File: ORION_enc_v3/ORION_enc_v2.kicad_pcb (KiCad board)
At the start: 2 copper layers, 24 x 31 mm, 21 parts, among them J1 Conn_01x01, J2 Conn_01x01, J3 Conn_01x01, J4 Conn_01x01, J5 Conn_01x01, J6 Conn_01x01, J7 Conn_01x01, U1 AS5047D

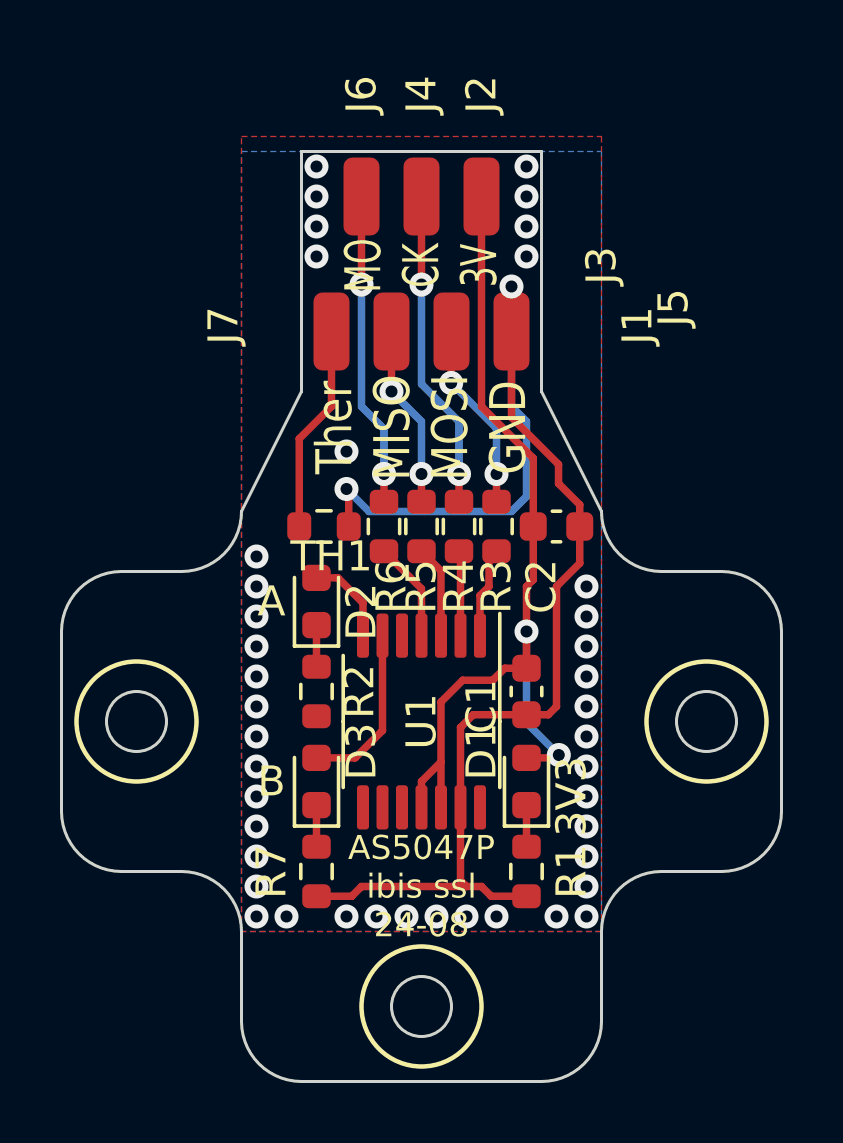
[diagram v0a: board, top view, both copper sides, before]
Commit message: 全てを追加
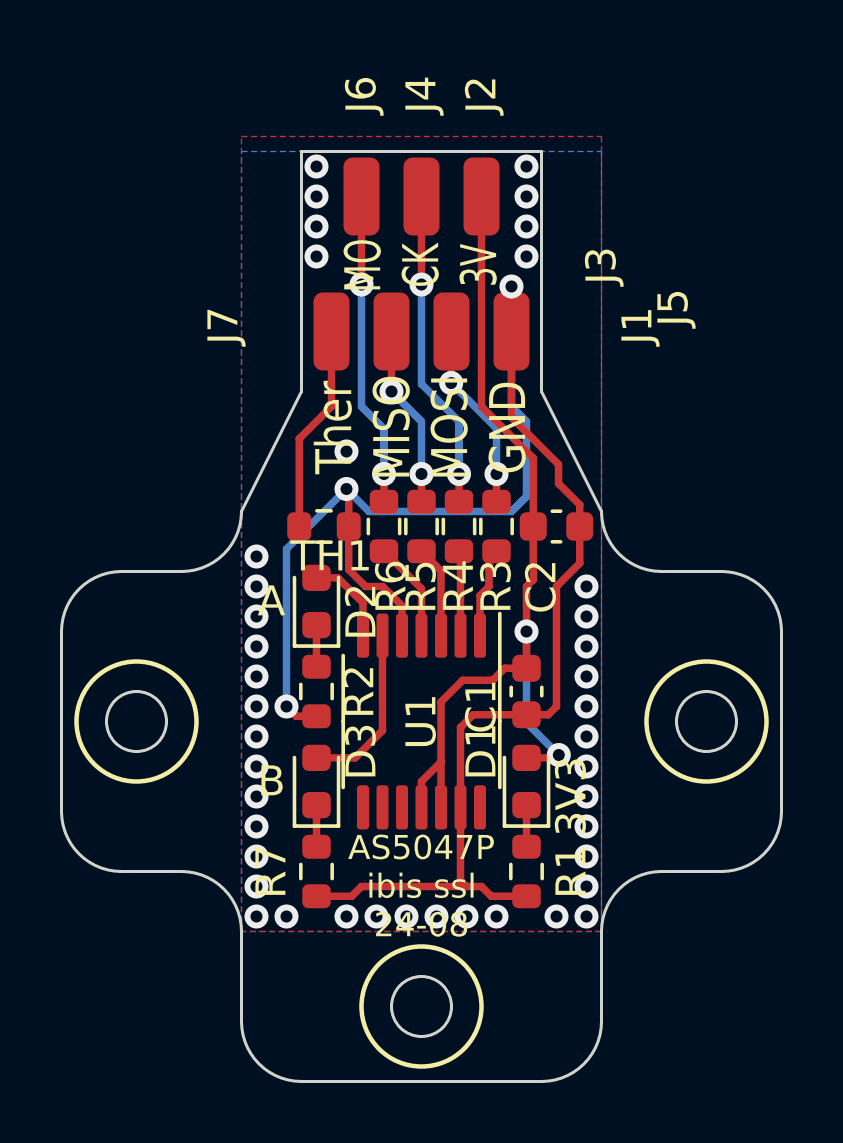
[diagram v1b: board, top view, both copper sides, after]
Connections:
- U1 pad 5: unconnected-(U1-Pad5) -> GND
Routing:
- net GND: track 46.7 -> 60.6 mm, vias 44 -> 45
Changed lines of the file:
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@@
   (net 12 "/MOSI")
   (net 13 "Net-(J7-Pad1)")
-  (net 14 "unconnected-(U1-Pad5)")
-  (net 15 "unconnected-(U1-Pad8)")
-  (net 16 "unconnected-(U1-Pad9)")
-  (net 17 "unconnected-(U1-Pad10)")
-  (net 18 "/OUT_A")
-  (net 19 "Net-(D3-Pad1)")
-  (net 20 "/OUT_B")
-  (net 21 "unconnected-(U1-Pad14)")
+  (net 14 "unconnected-(U1-Pad8)")
+  (net 15 "unconnected-(U1-Pad9)")
+  (net 16 "unconnected-(U1-Pad10)")
+  (net 17 "/OUT_A")
+  (net 18 "Net-(D3-Pad1)")
+  (net 19 "/OUT_B")
+  (net 20 "unconnected-(U1-Pad14)")
   (footprint "user:WireSoldingPad" (layer "F.Cu")
     (at 67 46.5 90)
@@
       (net 12 "/MOSI") (pinfunction "MOSI") (pintype "input"))
     (pad "5" smd roundrect (at -2.8625 0.65 270) (size 1.475 0.4) (layers "F.Cu" "F.Paste" "F.Mask") (roundrect_rratio 0.25)
-      (net 14 "unconnected-(U1-Pad5)") (pinfunction "TST") (pintype "input+no_connect"))
+      (net 2 "GND") (pinfunction "TST") (pintype "input"))
     (pad "6" smd roundrect (at -2.8625 1.3 270) (size 1.475 0.4) (layers "F.Cu" "F.Paste" "F.Mask") (roundrect_rratio 0.25)
-      (net 20 "/OUT_B") (pinfunction "B") (pintype "output"))
+      (net 19 "/OUT_B") (pinfunction "B") (pintype "output"))
     (pad "7" smd roundrect (at -2.8625 1.95 270) (size 1.475 0.4) (layers "F.Cu" "F.Paste" "F.Mask") (roundrect_rratio 0.25)
-      (net 18 "/OUT_A") (pinfunction "A") (pintype "output"))
+      (net 17 "/OUT_A") (pinfunction "A") (pintype "output"))
     (pad "8" smd roundrect (at 2.8625 1.95 270) (size 1.475 0.4) (layers "F.Cu" "F.Paste" "F.Mask") (roundrect_rratio 0.25)
-      (net 15 "unconnected-(U1-Pad8)") (pinfunction "W/PWM") (pintype "output+no_connect"))
+      (net 14 "unconnected-(U1-Pad8)") (pinfunction "W/PWM") (pintype "output+no_connect"))
     (pad "9" smd roundrect (at 2.8625 1.3 270) (size 1.475 0.4) (layers "F.Cu" "F.Paste" "F.Mask") (roundrect_rratio 0.25)
-      (net 16 "unconnected-(U1-Pad9)") (pinfunction "V") (pintype "output+no_connect"))
+      (net 15 "unconnected-(U1-Pad9)") (pinfunction "V") (pintype "output+no_connect"))
     (pad "10" smd roundrect (at 2.8625 0.65 270) (size 1.475 0.4) (layers "F.Cu" "F.Paste" "F.Mask") (roundrect_rratio 0.25)
-      (net 17 "unconnected-(U1-Pad10)") (pinfunction "U") (pintype "output+no_connect"))
+      (net 16 "unconnected-(U1-Pad10)") (pinfunction "U") (pintype "output+no_connect"))
     (pad "11" smd roundrect (at 2.8625 0 270) (size 1.475 0.4) (layers "F.Cu" "F.Paste" "F.Mask") (roundrect_rratio 0.25)
       (net 1 "+3V3") (pinfunction "VDD") (pintype "power_in"))
@@
       (net 2 "GND") (pinfunction "GND") (pintype "power_in"))
     (pad "14" smd roundrect (at 2.8625 -1.95 270) (size 1.475 0.4) (layers "F.Cu" "F.Paste" "F.Mask") (roundrect_rratio 0.25)
-      (net 21 "unconnected-(U1-Pad14)") (pinfunction "I/PWM") (pintype "output+no_connect"))
+      (net 20 "unconnected-(U1-Pad14)") (pinfunction "I/PWM") (pintype "output+no_connect"))
     (model "${KICAD6_3DMODEL_DIR}/Package_SO.3dshapes/TSSOP-14_4.4x5mm_P0.65mm.wrl"
       (offset (xyz 0 0 0))
@@
     (fp_line (start 0.8 -0.4125) (end 0.8 0.4125) (layer "F.Fab") (width 0.1))
     (pad "1" smd roundrect (at -0.825 0 270) (size 0.8 0.95) (layers "F.Cu" "F.Paste" "F.Mask") (roundrect_rratio 0.25)
-      (net 19 "Net-(D3-Pad1)") (pintype "passive"))
+      (net 18 "Net-(D3-Pad1)") (pintype "passive"))
     (pad "2" smd roundrect (at 0.825 0 270) (size 0.8 0.95) (layers "F.Cu" "F.Paste" "F.Mask") (roundrect_rratio 0.25)
       (net 2 "GND") (pintype "passive"))
@@
     (fp_line (start -0.8 0.4) (end 0.8 0.4) (layer "F.Fab") (width 0.1))
     (pad "1" smd roundrect (at -0.7875 0 90) (size 0.875 0.95) (layers "F.Cu" "F.Paste" "F.Mask") (roundrect_rratio 0.25)
-      (net 19 "Net-(D3-Pad1)") (pinfunction "K") (pintype "passive"))
+      (net 18 "Net-(D3-Pad1)") (pinfunction "K") (pintype "passive"))
     (pad "2" smd roundrect (at 0.7875 0 90) (size 0.875 0.95) (layers "F.Cu" "F.Paste" "F.Mask") (roundrect_rratio 0.25)
-      (net 20 "/OUT_B") (pinfunction "A") (pintype "passive"))
+      (net 19 "/OUT_B") (pinfunction "A") (pintype "passive"))
     (model "${KICAD6_3DMODEL_DIR}/LED_SMD.3dshapes/LED_0603_1608Metric.wrl"
       (offset (xyz 0 0 0))
@@
       (net 4 "Net-(D2-Pad1)") (pinfunction "K") (pintype "passive"))
     (pad "2" smd roundrect (at 0.7875 0 90) (size 0.875 0.95) (layers "F.Cu" "F.Paste" "F.Mask") (roundrect_rratio 0.25)
-      (net 18 "/OUT_A") (pinfunction "A") (pintype "passive"))
+      (net 17 "/OUT_A") (pinfunction "A") (pintype "passive"))
     (model "${KICAD6_3DMODEL_DIR}/LED_SMD.3dshapes/LED_0603_1608Metric.wrl"
       (offset (xyz 0 0 0))
@@
   (segment (start 73.568198 56.068198) (end 73.568198 55.431802) (width 0.25) (layer "F.Cu") (net 2))
   (segment (start 74.275 57.5) (end 74.275 56.775) (width 0.25) (layer "F.Cu") (net 2))
+  (segment (start 68.35 60.142462) (end 67.707538 59.5) (width 0.25) (layer "F.Cu") (net 2))
   (segment (start 66.5 56.25) (end 66.575 56.325) (width 0.25) (layer "F.Cu") (net 2))
+  (segment (start 64.825 63.825) (end 64.5 63.5) (width 0.25) (layer "F.Cu") (net 2))
   (segment (start 72 53.863604) (end 72 51) (width 0.25) (layer "F.Cu") (net 2))
+  (segment (start 67.136396 59.5) (end 66.575 58.938604) (width 0.25) (layer "F.Cu") (net 2))
   (segment (start 74.275 58.725) (end 74.275 57.5) (width 0.25) (layer "F.Cu") (net 2))
   (segment (start 73.5 59.5) (end 74.275 58.725) (width 0.25) (layer "F.Cu") (net 2))
   (segment (start 70.5 69.5) (end 71 69.5) (width 0.25) (layer "F.Cu") (net 2))
+  (segment (start 67.707538 59.5) (end 67.136396 59.5) (width 0.25) (layer "F.Cu") (net 2))
   (segment (start 72.5 63.775) (end 73.225 63.775) (width 0.25) (layer "F.Cu") (net 2))
   (segment (start 73.5 63.5) (end 73.5 59.5) (width 0.25) (layer "F.Cu") (net 2))
+  (segment (start 68.35 61.1375) (end 68.35 60.142462) (width 0.25) (layer "F.Cu") (net 2))
   (segment (start 66.675 69.825) (end 67 69.5) (width 0.25) (layer "F.Cu") (net 2))
+  (segment (start 66.575 58.938604) (end 66.575 57.5) (width 0.25) (layer "F.Cu") (net 2))
   (segment (start 73.225 63.775) (end 73.5 63.5) (width 0.25) (layer "F.Cu") (net 2))
   (segment (start 71 69.5) (end 71.325 69.825) (width 0.25) (layer "F.Cu") (net 2))
@@
   (segment (start 65.5 69.825) (end 66.675 69.825) (width 0.25) (layer "F.Cu") (net 2))
   (segment (start 74.275 56.775) (end 73.568198 56.068198) (width 0.25) (layer "F.Cu") (net 2))
+  (segment (start 65.5 63.825) (end 64.825 63.825) (width 0.25) (layer "F.Cu") (net 2))
   (segment (start 71.325 69.825) (end 72.5 69.825) (width 0.25) (layer "F.Cu") (net 2))
   (segment (start 67 69.5) (end 70.5 69.5) (width 0.25) (layer "F.Cu") (net 2))
@@
   (via (at 71.5 70.5) (size 0.8) (drill 0.4) (layers "F.Cu" "B.Cu") (free) (net 2))
   (via (at 64.5 70.5) (size 0.8) (drill 0.4) (layers "F.Cu" "B.Cu") (free) (net 2))
+  (via (at 64.5 63.5) (size 0.8) (drill 0.4) (layers "F.Cu" "B.Cu") (net 2))
   (via (at 63.5 66.5) (size 0.8) (drill 0.4) (layers "F.Cu" "B.Cu") (free) (net 2))
   (via (at 74.5 63.5) (size 0.8) (drill 0.4) (layers "F.Cu" "B.Cu") (free) (net 2))
@@
   (segment (start 72 57) (end 67.25 57) (width 0.25) (layer "B.Cu") (net 2))
   (segment (start 72.5 54) (end 72.5 56.5) (width 0.25) (layer "B.Cu") (net 2))
+  (segment (start 64.5 63.5) (end 64.5 58.25) (width 0.25) (layer "B.Cu") (net 2))
   (segment (start 72 49.5) (end 72 53.5) (width 0.25) (layer "B.Cu") (net 2))
   (segment (start 72.5 56.5) (end 72 57) (width 0.25) (layer "B.Cu") (net 2))
+  (segment (start 64.5 58.25) (end 66.5 56.25) (width 0.25) (layer "B.Cu") (net 2))
   (segment (start 72 53.5) (end 72.5 54) (width 0.25) (layer "B.Cu") (net 2))
   (segment (start 72.5 66.7875) (end 72.5 68.175) (width 0.25) (layer "F.Cu") (net 3))
@@
   (segment (start 64.925 57.5) (end 64.925 54.575) (width 0.25) (layer "F.Cu") (net 13))
   (segment (start 66 53.5) (end 66 51) (width 0.25) (layer "F.Cu") (net 13))
-  (segment (start 67.05 60.05) (end 67.05 61.1375) (width 0.25) (layer "F.Cu") (net 18))
-  (segment (start 66.2125 59.2125) (end 67.05 60.05) (width 0.25) (layer "F.Cu") (net 18))
-  (segment (start 65.5 59.2125) (end 66.2125 59.2125) (width 0.25) (layer "F.Cu") (net 18))
-  (segment (start 65.5 66.7875) (end 65.5 68.175) (width 0.25) (layer "F.Cu") (net 19))
-  (segment (start 65.5 65.2125) (end 66.7875 65.2125) (width 0.25) (layer "F.Cu") (net 20))
-  (segment (start 66.7875 65.2125) (end 67.7 64.3) (width 0.25) (layer "F.Cu") (net 20))
-  (segment (start 67.7 64.3) (end 67.7 61.1375) (width 0.25) (layer "F.Cu") (net 20))
+  (segment (start 67.05 60.05) (end 67.05 61.1375) (width 0.25) (layer "F.Cu") (net 17))
+  (segment (start 66.2125 59.2125) (end 67.05 60.05) (width 0.25) (layer "F.Cu") (net 17))
+  (segment (start 65.5 59.2125) (end 66.2125 59.2125) (width 0.25) (layer "F.Cu") (net 17))
+  (segment (start 65.5 66.7875) (end 65.5 68.175) (width 0.25) (layer "F.Cu") (net 18))
+  (segment (start 65.5 65.2125) (end 66.7875 65.2125) (width 0.25) (layer "F.Cu") (net 19))
+  (segment (start 66.7875 65.2125) (end 67.7 64.3) (width 0.25) (layer "F.Cu") (net 19))
+  (segment (start 67.7 64.3) (end 67.7 61.1375) (width 0.25) (layer "F.Cu") (net 19))
   (zone (net 2) (net_name "GND") (layer "F.Cu") (hatch edge 0.508)
     (connect_pads (clearance 0.2))
